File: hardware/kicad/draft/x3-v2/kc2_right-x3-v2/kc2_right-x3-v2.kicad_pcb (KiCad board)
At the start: 2 copper layers, 163.7 x 122.5 mm, 92 parts, among them SW1 KEY_01, SW10 KEY_10, SW11 KEY_11, SW12 KEY_12, SW13 KEY_13, SW14 KEY_14, SW15 KEY_15, SW16 KEY_16, SW17 KEY_17, SW18 KEY_18, SW19 KEY_19, SW2 KEY_02, SW20 KEY_20, SW21 KEY_21, SW22 KEY_22, SW23 KEY_23, SW24 KEY_24, SW25 KEY_25, SW26 KEY_26, SW27 KEY_27, SW28 KEY_28, SW29 KEY_29, SW3 KEY_03, SW30 KEY_30, SW31 KEY_31, SW32 KEY_32, SW33 KEY_33, SW34 KEY_34, SW35 KEY_35, SW36 KEY_36, SW37 KEY_37, SW38 KEY_38, SW39 KEY_39, SW4 KEY_04, SW5 KEY_05, SW6 KEY_06, SW7 KEY_07, SW8 KEY_08, SW9 KEY_09, U1 nice!nano_v2_socket_24pin

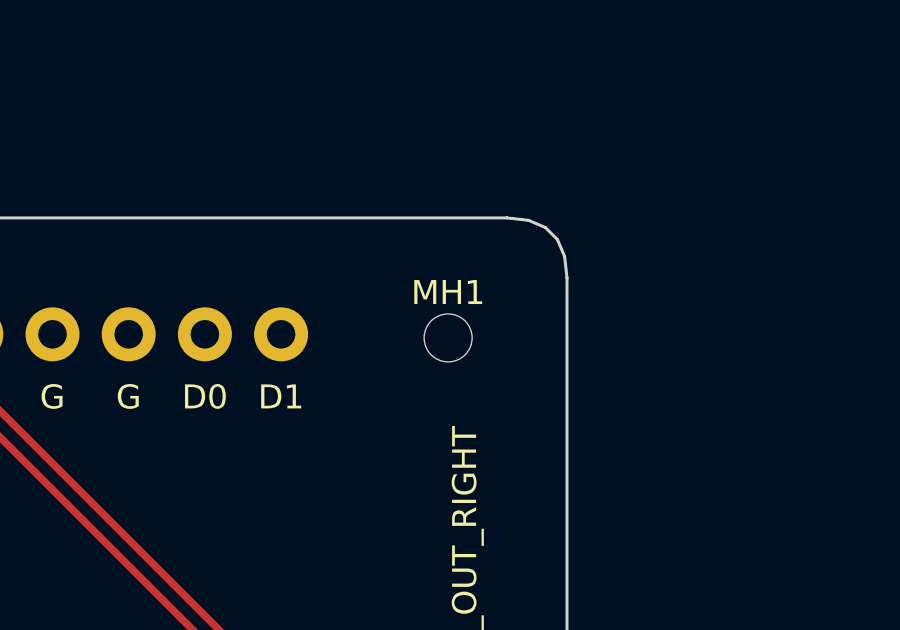
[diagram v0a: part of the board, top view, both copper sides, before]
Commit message: wip(x3-v2): refresh P2 mounts and artifacts
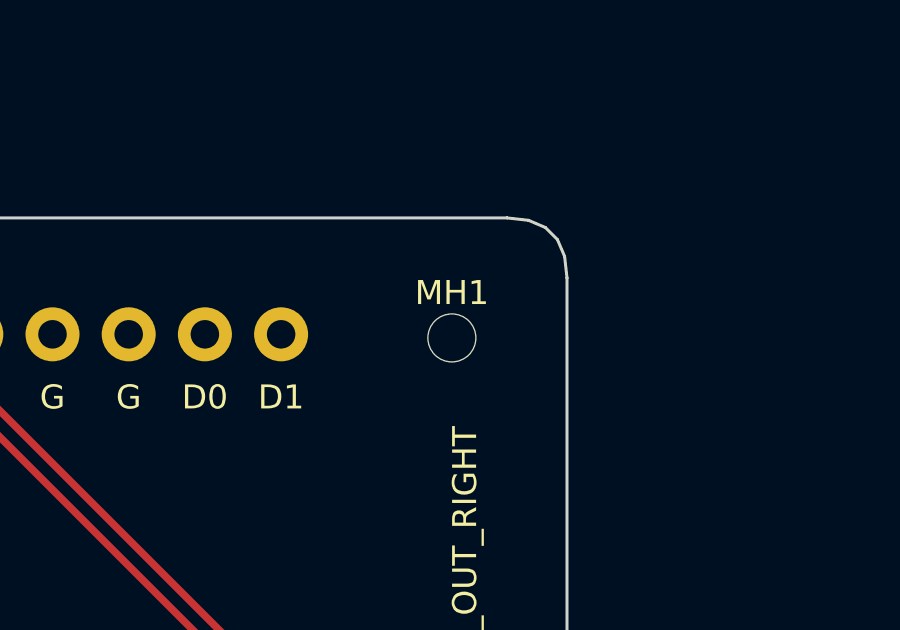
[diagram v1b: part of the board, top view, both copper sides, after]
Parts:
- moved MH1 0.12 mm to (97.1, 43.2)
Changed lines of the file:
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@@
 	(footprint "MH_M1.4_NPTH_1.60"
 		(layer "F.Cu")
-		(at 96.9375 43.25)
+		(at 97.0625 43.25)
 		(descr "KC2 X3 V2 M1.4 service mounting hole, 1.60 mm copper-free NPTH")
 		(tags "KC2 X3 V2 M1.4 mounting NPTH copper-free")
